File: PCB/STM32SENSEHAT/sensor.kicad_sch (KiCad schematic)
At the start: 18 parts, among them J11 Conn_01x02_Pin, U4 BME280, U6 LTR-303ALS-01

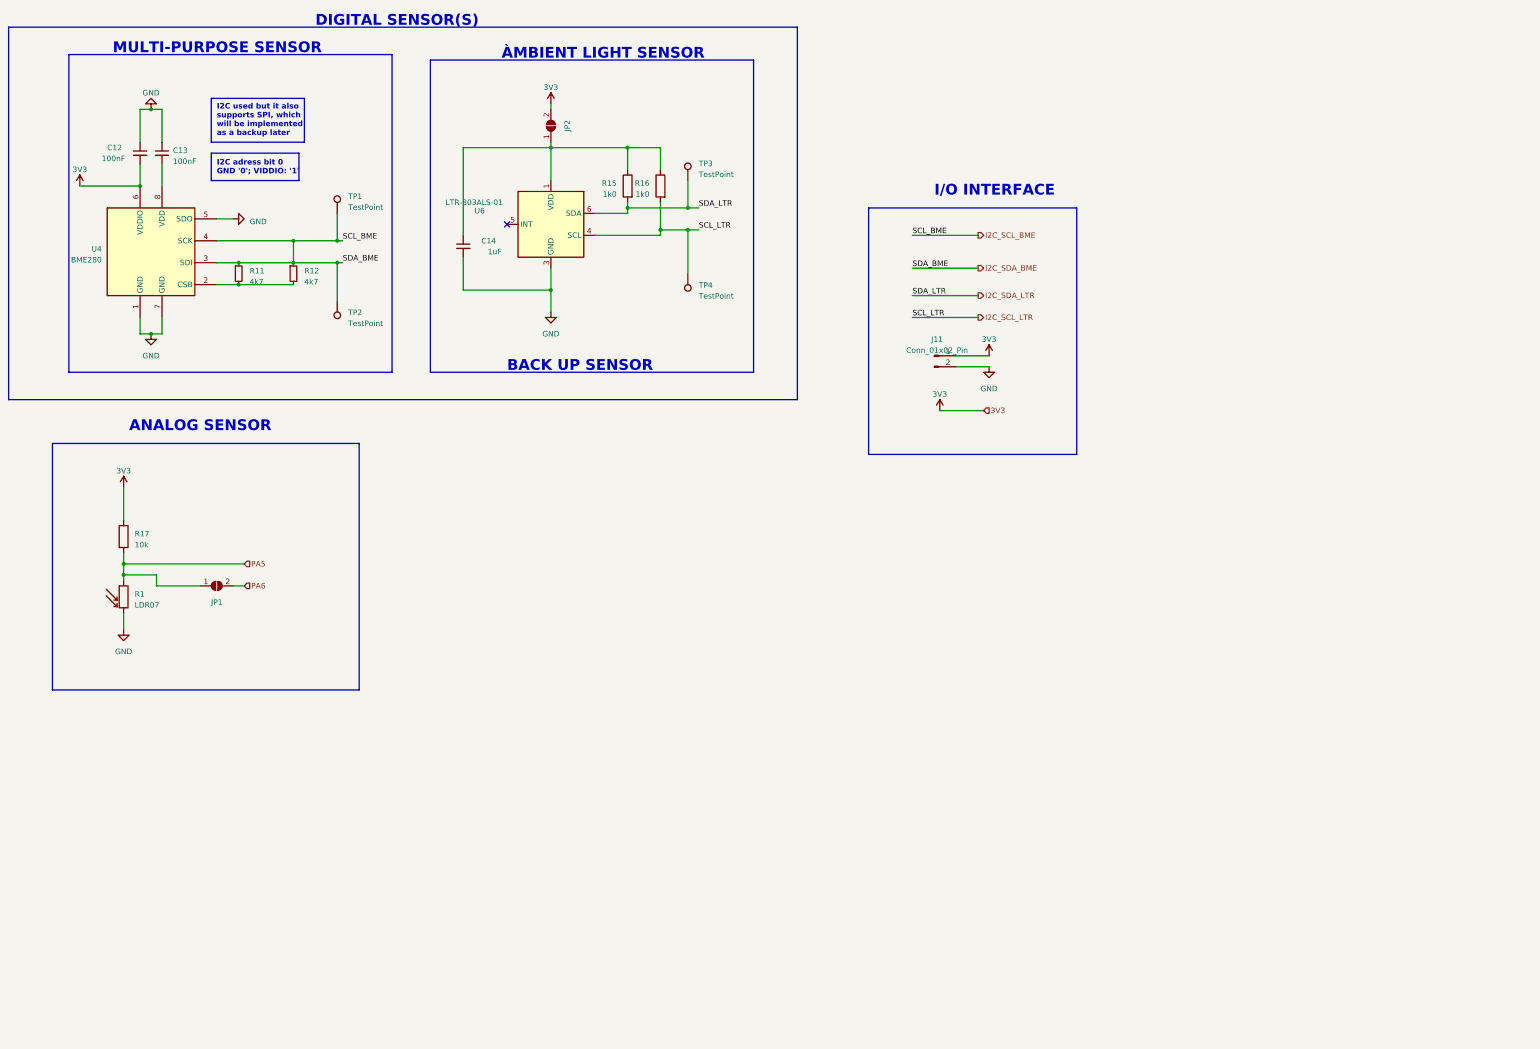
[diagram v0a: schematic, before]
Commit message: Protectuion features added to all schematica
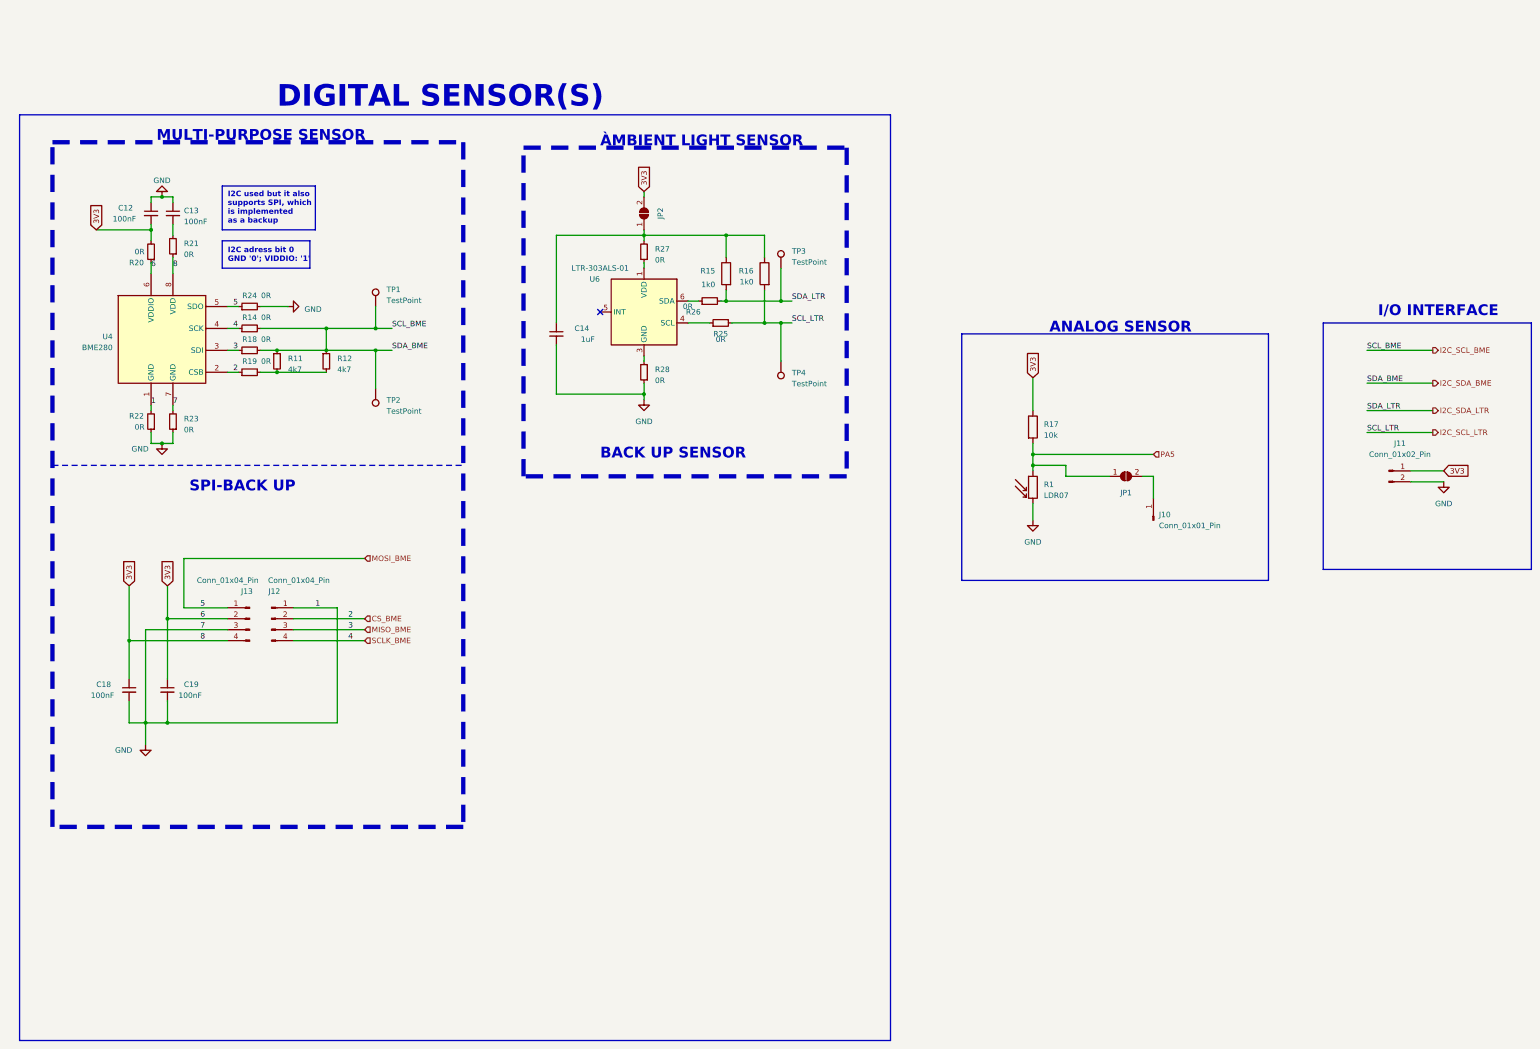
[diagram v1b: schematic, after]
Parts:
- added C18, C19: 100nF, symbol Device:C_Small
- added J10: Conn_01x01_Pin, symbol Connector:Conn_01x01_Pin
- added J12, J13: Conn_01x04_Pin, symbol Connector:Conn_01x04_Pin
- added R14, R18, R19, R20, R21, R22, R23, R24, R25, R26, R27, R28: 0R, symbol Device:R_Small
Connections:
- net GND: now also C18.2, C19.2, J12.1 (Pin_1), J13.3 (Pin_3), R22.1, R22.2, R23.1, R23.2, R24.2, R28.1; no longer U4.5 (SDO), U6.3 (GND)
- net I2C_SCL_BME: now also R14.2, R18.2; no longer U4.3 (SDI), U4.4 (SCK)
- net I2C_SCL_LTR: now also R25.2; no longer U6.4 (SCL)
- net I2C_SDA_LTR: now also R26.2; no longer U6.6 (SDA)
- net at R11.2, R12.2: now also R19.2; no longer U4.2 (CSB)
- net at C13.2: now also R21.2; no longer U4.8 (VDD)
- net at C14.1, JP2.1 (A), R15.1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: now also R27.2; no longer U6.1 (VDD)
- net PA6: no longer names the net of JP1.2 (B)
- net PA6: now also J10.1 (Pin_1)
- net VCC renamed 3V3
- net 3V3: now also U4.8 (VDD), C18.1, C19.1, J13.2 (Pin_2), J13.4 (Pin_4), R20.1, R20.2, R21.1
- new net: R26.1, U6.6 (SDA)
- new net: R27.1, U6.1 (VDD)
- new net: R28.2, U6.3 (GND)
- new net: R25.1, U6.4 (SCL)
- new net CS_BME: J12.2 (Pin_2), R19.1, U4.2 (CSB)
- new net MISO_BME: J12.3 (Pin_3), R18.1, U4.3 (SDI)
- new net MOSI_BME: J13.1 (Pin_1), R24.1, U4.5 (SDO)
- new net SCLK_BME: J12.4 (Pin_4), R14.1, U4.4 (SCK)
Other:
- note added: "I2C used but it also supports SPI, which is implemented as a backup"
- note added: "SPI-BACK UP"
- note removed: "I2C used but it also supports SPI, which will be implemented as a backup later"
- moved on the sheet: C12, C13, C14, J11, JP1, JP2, R1, R11, R12, R15, R16, R17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
